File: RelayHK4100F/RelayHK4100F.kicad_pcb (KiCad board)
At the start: 2 copper layers, 31.7 x 15.2 mm, 3 parts, among them J1 Conn_01x05, K1 Y14x-1C-xxDS

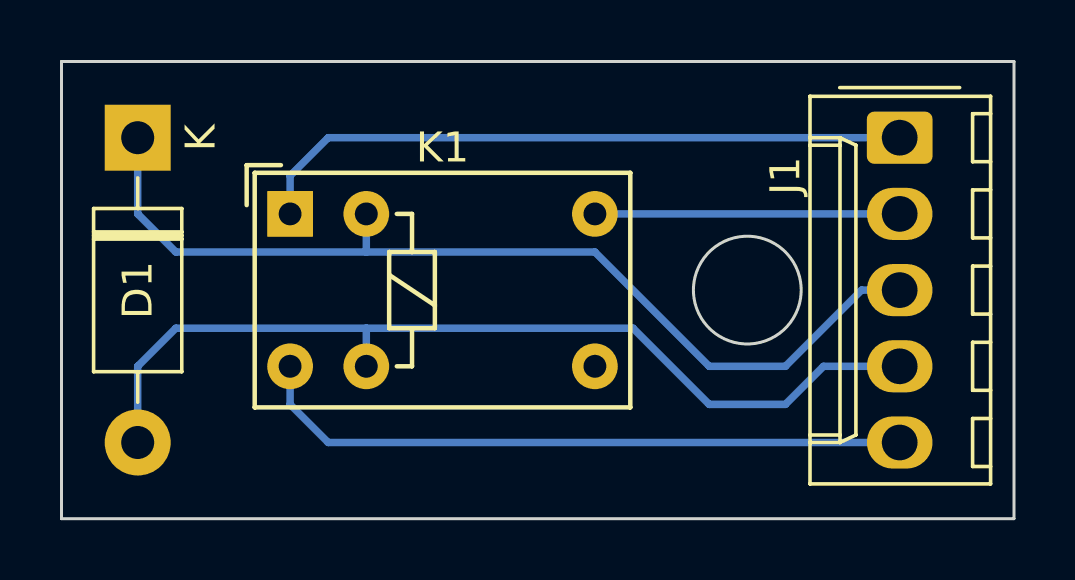
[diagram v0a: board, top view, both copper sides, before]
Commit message: Proyecto relay
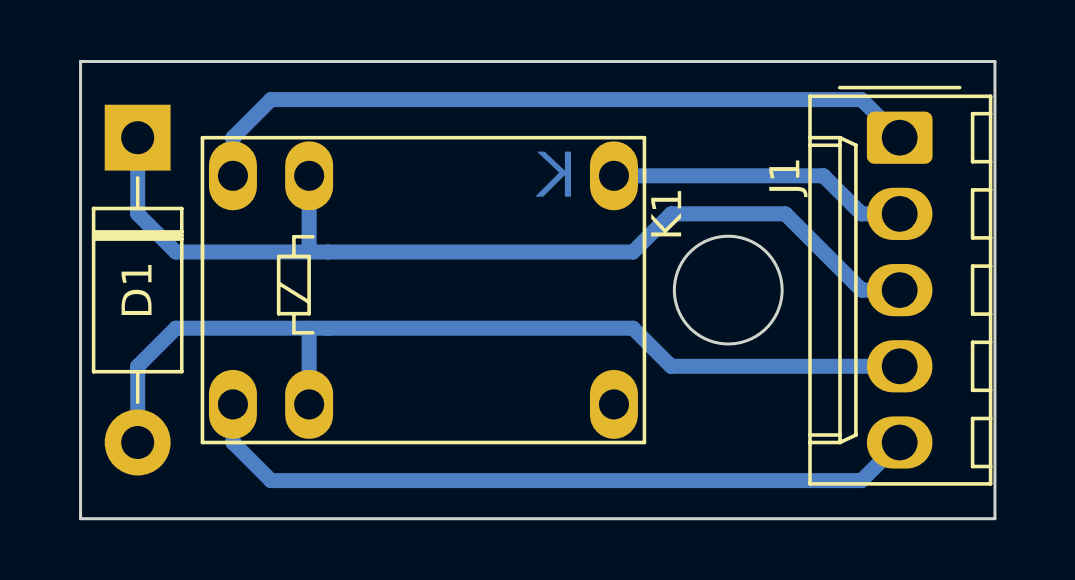
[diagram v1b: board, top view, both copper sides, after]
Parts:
- K1: value Y14x-1C-xxDS -> TIANBO-HJR-4102-L; footprint Relay_THT:Relay_SPDT_HsinDa_Y14 -> Relay_THT:Relay_SPDT_HJR-4102
- moved K1 10.9 mm to (130.2, 82.5), turned to -90 degrees
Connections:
- D1 pad 1: Net-(D1-Pad1) -> /DN
- D1 pad 2: Net-(D1-Pad2) -> /DP
- J1 pad 1: Net-(J1-Pad1) -> /NO
- J1 pad 2: Net-(J1-Pad2) -> /COM
- J1 pad 3: Net-(D1-Pad1) -> /DN
- J1 pad 4: Net-(D1-Pad2) -> /DP
- J1 pad 5: Net-(J1-Pad5) -> /NC
- K1 pad 5: Net-(J1-Pad2) -> /DN
- K1 pad 6: Net-(J1-Pad2) -> /NO
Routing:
- net /DN: track 0.00 -> 32.6 mm
- net Net-(D1-Pad1): track 32.4 -> 0.00 mm
- net /DP: track 0.00 -> 31.5 mm
- net Net-(D1-Pad2): track 31.3 -> 0.00 mm
- net /NO: track 0.00 -> 24.5 mm
- net /NC: track 0.00 -> 24.5 mm
- net Net-(J1-Pad5): track 22.1 -> 0.00 mm
- net Net-(J1-Pad1): track 22.1 -> 0.00 mm
- net Net-(J1-Pad2): track 10.2 -> 0.00 mm
- net /COM: track 0.00 -> 10.1 mm
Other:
- board size 31.7 x 15.2 mm -> 30.5 x 15.2 mm
- board text added: "K"
